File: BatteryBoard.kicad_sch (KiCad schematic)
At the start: 19 parts, among them J1 Keystone-1042, J11 Conn_01x12_MountingPin, J14 Conn_01x04, J15 Conn_01x04, J2 Keystone-1042, J3 Keystone-1042, J4 Keystone-1042, J5 Keystone-1042, J6 Keystone-1042, SW1 SW_SPST, SW2 SW_SPST, SW3 SW_SPST, SW4 SW_SPST

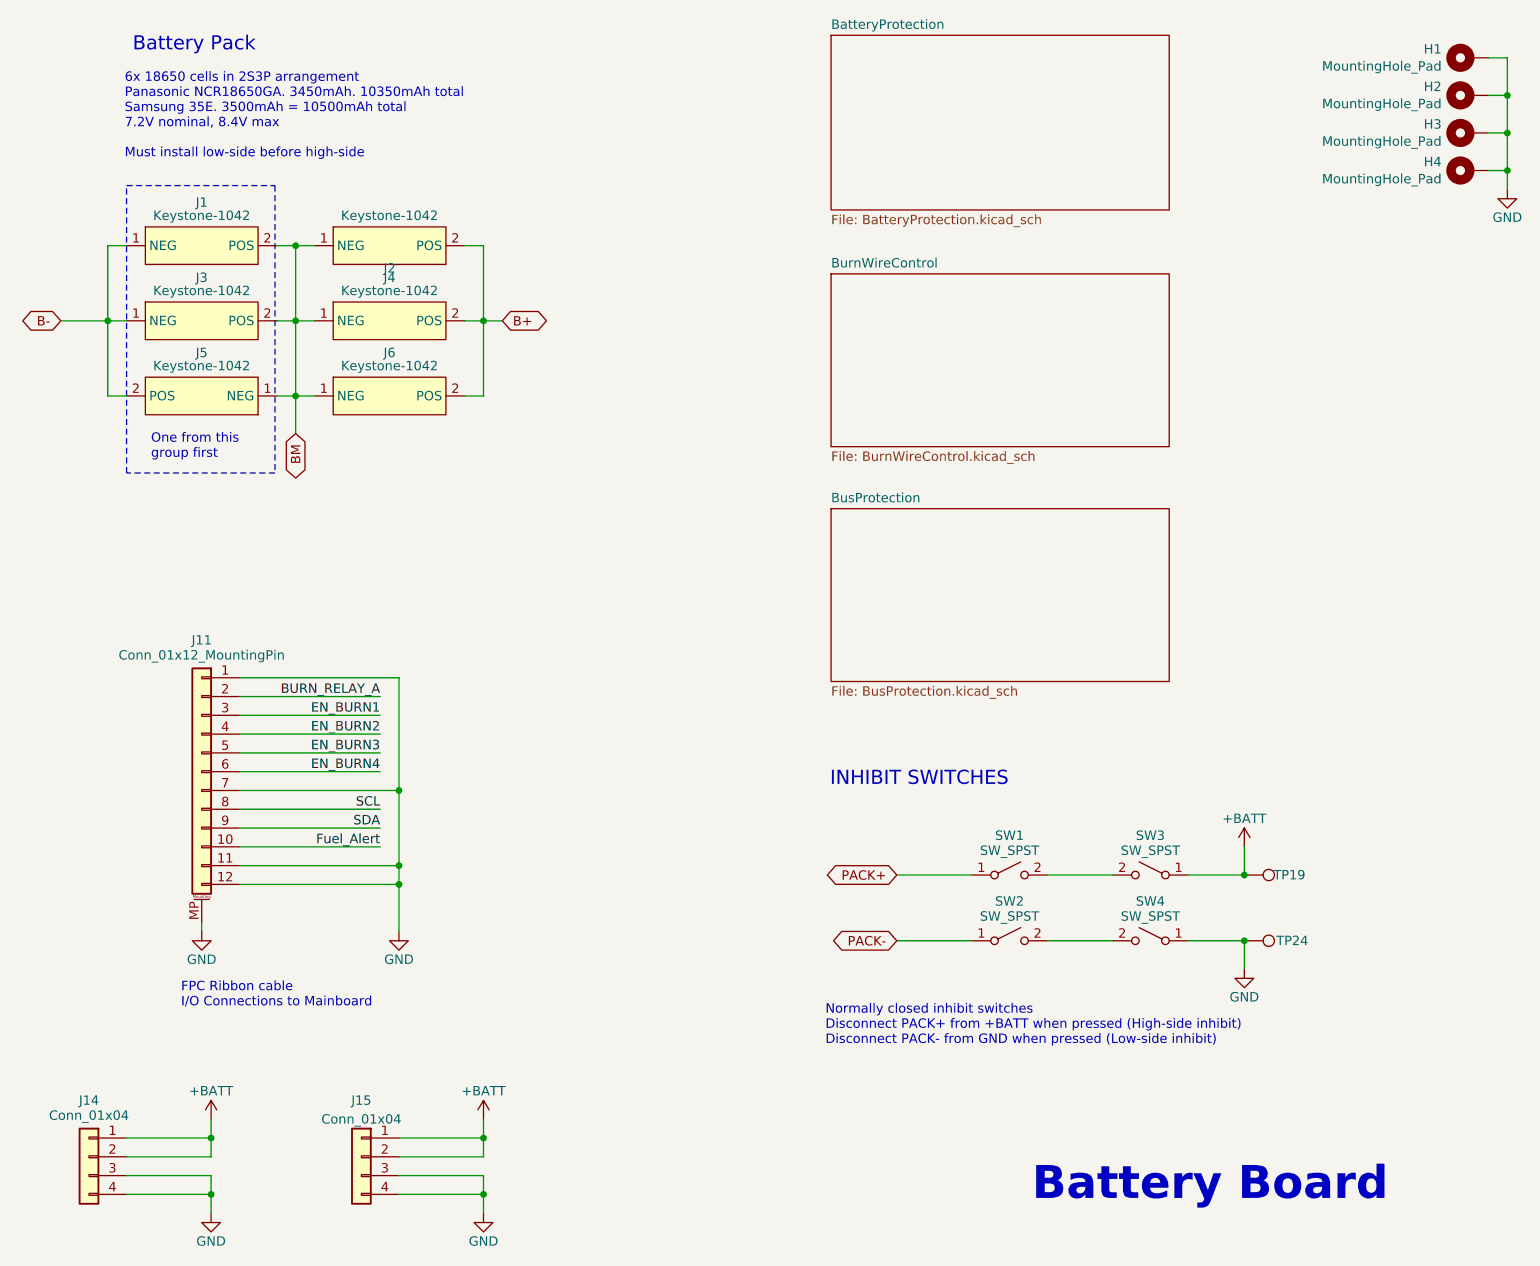
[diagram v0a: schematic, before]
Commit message: Finish v1 schematic
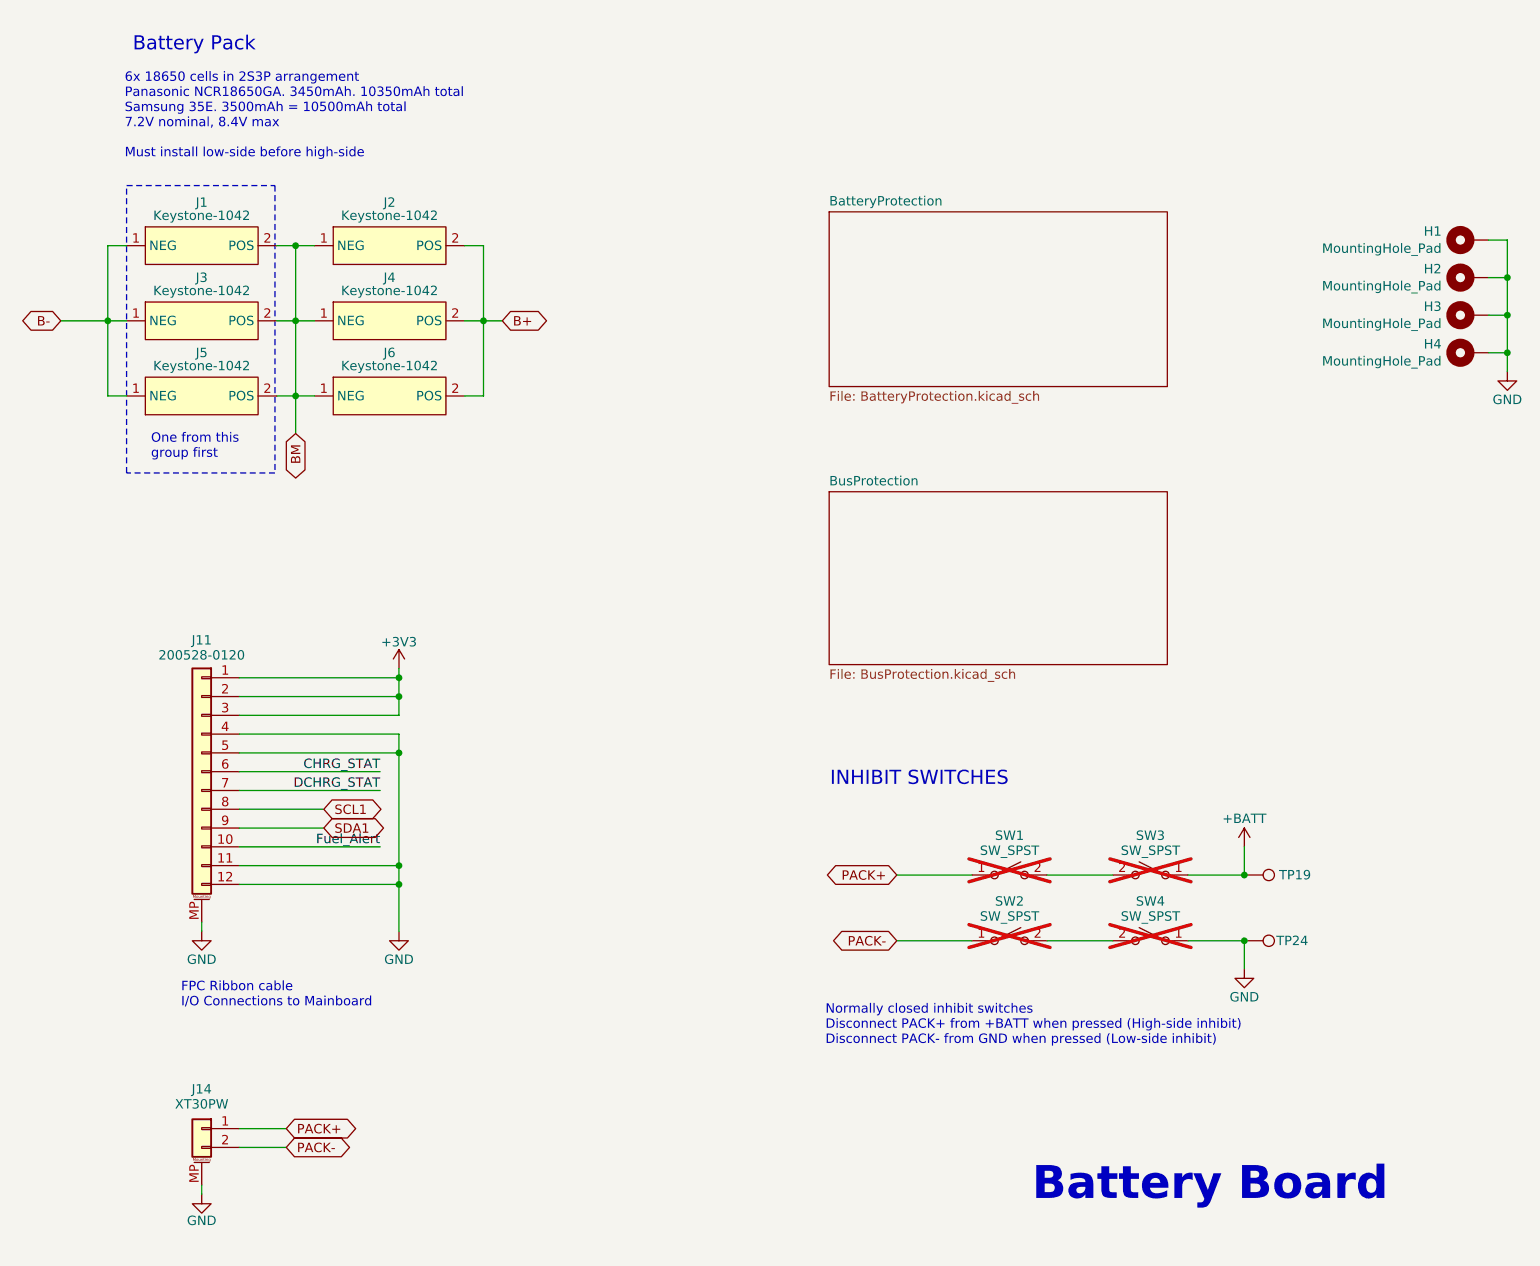
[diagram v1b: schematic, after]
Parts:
- removed J15: Conn_01x04, symbol Connector_Generic:Conn_01x04
- H1, H2, H3, H4: footprint custom-footprints:MountingHole_3.2mm_M3_DIN965_PadMOD -> BatteryBoard:MountingHole
- J1, J2, J3, J4, J5, J6: footprint KEYSTONE-1042 -> BatteryBoard:Keystone_1042
- J11: value Conn_01x12_MountingPin -> 200528-0120; footprint (none) -> Connector_FFC-FPC:Molex_200528-0120_1x12-1MP_P1.00mm_Horizontal
- J14: value Conn_01x04 -> XT30PW; footprint (none) -> BatteryBoard:AMASS_XT30PW-M; symbol Connector_Generic:Conn_01x04 -> Connector_Generic_MountingPin:Conn_01x02_MountingPin
- SW1, SW2, SW3, SW4: now not fitted
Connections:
- net EN_BURN1 is gone; now on net +3V3: J11.3 (Pin_3)
- net EN_BURN2 is gone; now on net GND: J11.4 (Pin_4)
- net EN_BURN3 is gone; now on net GND: J11.5 (Pin_5)
- net +BATT: no longer J14.1 (Pin_1), J14.2 (Pin_2)
- net B-: now also J5.1 (NEG); no longer J5.2 (POS)
- net BM: now also J5.2 (POS); no longer J5.1 (NEG)
- net GND: now also J14.MP (MountPin); no longer J11.1 (Pin_1), J11.7 (Pin_7), J14.3 (Pin_3), J14.4 (Pin_4)
- net PACK+: now also J14.1 (Pin_1)
- net PACK-: now also J14.2 (Pin_2)
- net BURN_RELAY_A renamed +3V3
- net +3V3: now also J11.1 (Pin_1)
- net EN_BURN4 renamed CHRG_STAT
- net SCL renamed SCL1
- net SDA renamed SDA1
- new net DCHRG_STAT: J11.7 (Pin_7)
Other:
- removed sheet BurnWireControl
- moved on the sheet: H1, H2, H3, H4, J5
